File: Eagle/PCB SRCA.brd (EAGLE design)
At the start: 160 x 100 mm, 77 parts, among them IC1 DSPIC30F4011-30I_P, IC2 LM324LVIDR, IC3 LM35DZ_NOPB, IC4 FT232RL-REEL, J1 TBL002A-350-03GR-2OR, J2 TBL002A-350-03GR-2OR, J3 TBL002A-350-03GR-2OR, J4 44914-0801, J5 TBL002A-350-03GR-2OR, J6 44914-0401, Q1 TIP41C, T1 2N3904, T2 2N3904, T3 2N3904, T4 2N3904, T5 2N3904, T6 2N3904, T7 2N3904, T8 2N3904, T9 2N3904, U1 LD1117S33TR

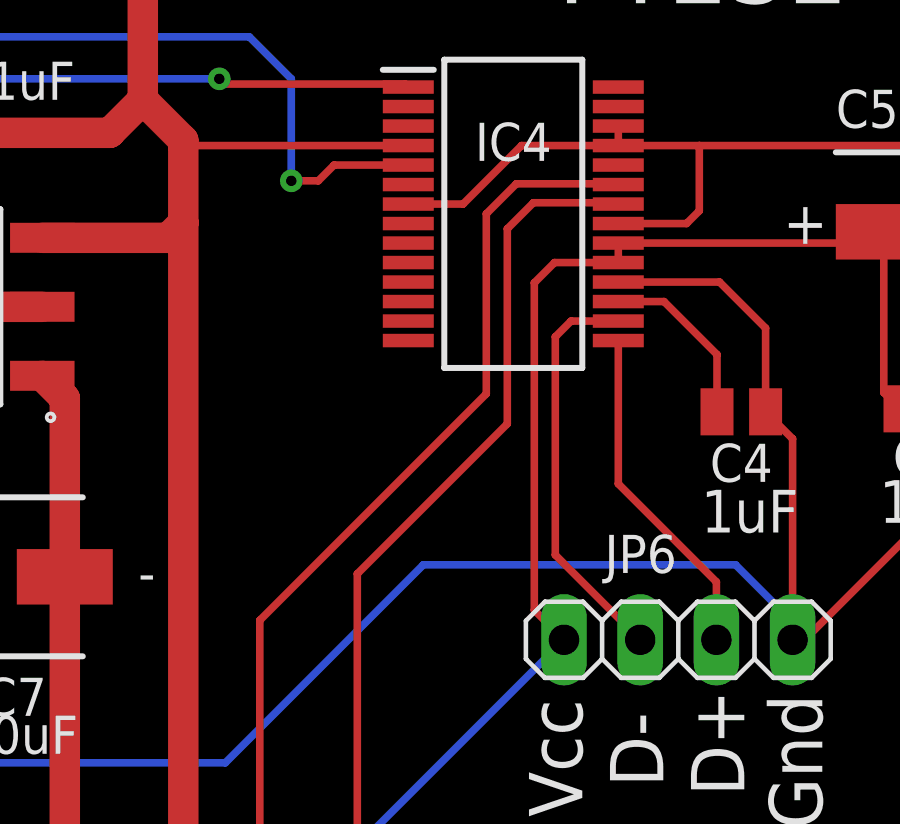
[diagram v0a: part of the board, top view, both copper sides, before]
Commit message: 23-09-2021
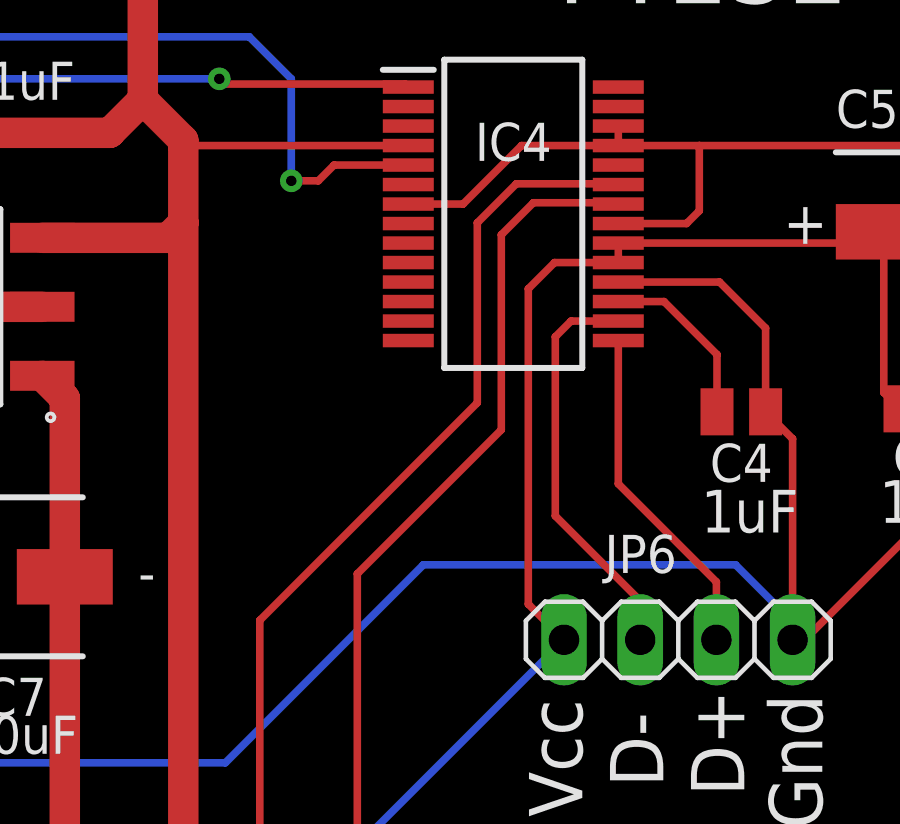
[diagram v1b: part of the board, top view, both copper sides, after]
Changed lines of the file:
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@@
 <drawing>
 <settings>
-<setting alwaysvectorfont="no"/>
+<setting alwaysvectorfont="yes"/>
 <setting verticaltext="up"/>
 </settings>
@@
 </layers>
 <board>
-<fusionsync huburn="a.YnVzaW5lc3M6Z21haWwxODU1MTgw" projecturn="a.YnVzaW5lc3M6Z21haWwxODU1MTgwIzIwMjEwODI0NDM3MjIwNDA2" f3durn="urn:adsk.wipprod:dm.lineage:9RdnEizDSZWnVXfx1H3Ocg" pcbguid="" lastpulledtime="" lastsyncedchangeguid="" latestrevisionid="20cc03f1-af99-4a4c-a276-f269cff5e179" lastsyncedrevisionid="20cc03f1-af99-4a4c-a276-f269cff5e179" lastboardhashguid="1d953e68-588c-0330-f4bb-c947bb569c06" lastpushedtime="2021-09-06T21:43:07Z" linktopcb3d="true"/>
+<fusionsync huburn="a.YnVzaW5lc3M6Z21haWwxODU1MTgw" projecturn="a.YnVzaW5lc3M6Z21haWwxODU1MTgwIzIwMjEwODI0NDM3MjIwNDA2" f3durn="urn:adsk.wipprod:dm.lineage:9RdnEizDSZWnVXfx1H3Ocg" pcbguid="" lastpulledtime="" lastsyncedchangeguid="" latestrevisionid="c4a1ce47-2d88-4aa0-bed6-f5c6ff134eef" lastsyncedrevisionid="c4a1ce47-2d88-4aa0-bed6-f5c6ff134eef" lastboardhashguid="45040a8e-f6d4-4a60-a59d-9d538ec767cb" lastpushedtime="2021-09-06T22:51:12Z" linktopcb3d="true"/>
 <plain>
 <text x="9.69" y="29.4" size="1.778" layer="25">MCLR</text>
@@
 <wire x1="133.1" y1="38.275" x2="133.1" y2="38.925" width="0.254" layer="1"/>
 <wire x1="133.1" y1="38.275" x2="130.975" y2="38.275" width="0.254" layer="1"/>
-<wire x1="130.975" y1="38.275" x2="130.3" y2="37.6" width="0.254" layer="1"/>
-<wire x1="130.3" y1="37.6" x2="130.3" y2="26.69" width="0.254" layer="1"/>
-<wire x1="130.3" y1="26.69" x2="131.29" y2="25.7" width="0.254" layer="1"/>
+<wire x1="130.975" y1="38.275" x2="130.1" y2="37.4" width="0.254" layer="1"/>
+<wire x1="130.1" y1="37.4" x2="130.1" y2="26.89" width="0.254" layer="1"/>
+<wire x1="130.1" y1="26.89" x2="131.29" y2="25.7" width="0.254" layer="1"/>
 <wire x1="126.1" y1="42.175" x2="118.6" y2="42.175" width="0.254" layer="1"/>
 <wire x1="94.5" y1="34.7" x2="96.48" y2="41.68" width="0.254" layer="1"/>
@@
 <contactref element="JP6" pad="2"/>
 <contactref element="IC4" pad="16"/>
-<wire x1="133.83" y1="25.7" x2="131" y2="28.53" width="0.254" layer="1"/>
-<wire x1="131" y1="28.53" x2="131" y2="35.8" width="0.254" layer="1"/>
+<wire x1="133.83" y1="25.7" x2="133.73" y2="25.8" width="0.254" layer="1"/>
+<wire x1="133.73" y1="27.1" x2="133.73" y2="25.8" width="0.254" layer="1"/>
+<wire x1="133.73" y1="27.1" x2="131" y2="29.83" width="0.254" layer="1"/>
+<wire x1="131" y1="29.83" x2="131" y2="35.8" width="0.254" layer="1"/>
 <wire x1="131" y1="35.8" x2="131.525" y2="36.325" width="0.254" layer="1"/>
 <wire x1="131.525" y1="36.325" x2="133.1" y2="36.325" width="0.254" layer="1"/>
@@
 <contactref element="IC4" pad="23"/>
 <contactref element="LED7" pad="1"/>
-<wire x1="128.7" y1="39.9" x2="129.7" y2="40.9" width="0.254" layer="1"/>
+<wire x1="128.4" y1="39.6" x2="129.7" y2="40.9" width="0.254" layer="1"/>
 <wire x1="133.075" y1="40.9" x2="133.1" y2="40.875" width="0.254" layer="1"/>
 <wire x1="129.7" y1="40.9" x2="133.075" y2="40.9" width="0.254" layer="1"/>
 <wire x1="121.15" y1="3.1" x2="121.15" y2="26.35" width="0.254" layer="1"/>
-<wire x1="128.7" y1="33.9" x2="128.7" y2="39.9" width="0.254" layer="1"/>
-<wire x1="121.15" y1="26.35" x2="128.7" y2="33.9" width="0.254" layer="1"/>
+<wire x1="128.4" y1="33.6" x2="128.4" y2="39.6" width="0.254" layer="1"/>
+<wire x1="121.15" y1="26.35" x2="128.4" y2="33.6" width="0.254" layer="1"/>
 </signal>
 <signal name="N$18">
@@
 <wire x1="115.607" y1="1.143" x2="123.6" y2="1.143" width="0.254" layer="1"/>
 <wire x1="123.6" y1="1.143" x2="124.4" y2="1.943" width="0.254" layer="1"/>
-<wire x1="124.4" y1="27.9" x2="129.4" y2="32.9" width="0.254" layer="1"/>
-<wire x1="129.4" y1="32.9" x2="129.4" y2="39.4" width="0.254" layer="1"/>
-<wire x1="129.4" y1="39.4" x2="130.269" y2="40.269" width="0.254" layer="1"/>
+<wire x1="124.4" y1="27.9" x2="129.2" y2="32.7" width="0.254" layer="1"/>
+<wire x1="129.2" y1="32.7" x2="129.2" y2="39.2" width="0.254" layer="1"/>
+<wire x1="129.2" y1="39.2" x2="130.269" y2="40.269" width="0.254" layer="1"/>
 <wire x1="133.056" y1="40.269" x2="133.1" y2="40.225" width="0.254" layer="1"/>
 <wire x1="124.4" y1="1.943" x2="124.4" y2="27.9" width="0.254" layer="1"/>
